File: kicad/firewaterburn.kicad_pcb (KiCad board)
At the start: 2 copper layers, 159.6 x 104.7 mm, 85 parts, among them J1 AudioJack2_SwitchT, J2 AudioJack2_SwitchT, J3 AudioJack2_SwitchT, J4 AudioJack2_SwitchT, J5 AudioJack2_SwitchT, J6 AudioJack2_SwitchT, J7 R61529 LCD, J9 Conn_01x03, P1 USB_C_Plug_USB2.0, Q1 DMN61D9UWQ-13, Q2 DMP31D0U-7, Q3 SS8050-G, Q4 SS8050-G, Q6 DMN2004WK-7, SW1 SW_MEC_5G, SW2 SW_MEC_5G, U1 RT9471GQW, U2 MCP1663T-E/MNY, U3 MCP1603-330I/MC, U4 ESP32-S3-Rx, U5 CP2102N-Axx-xQFN28

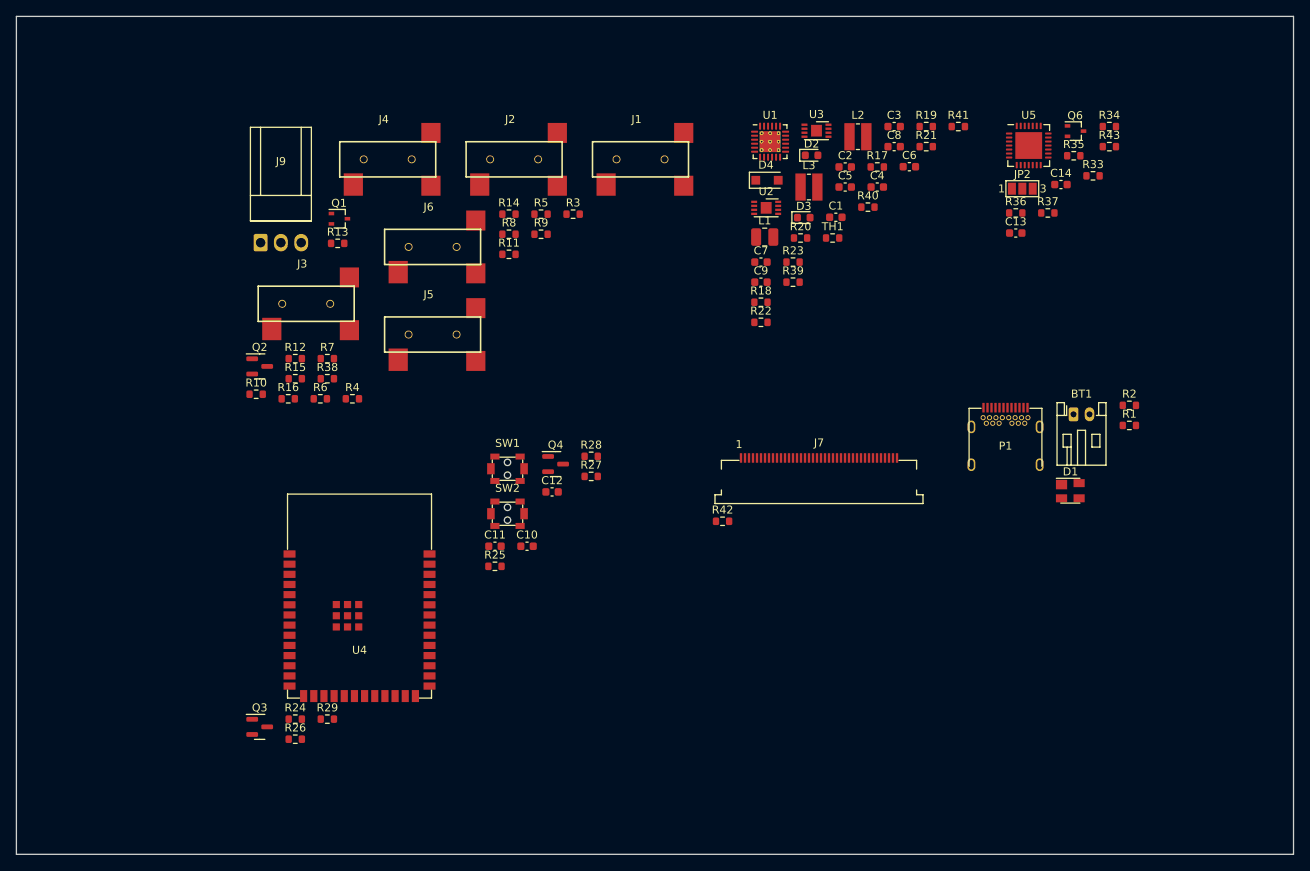
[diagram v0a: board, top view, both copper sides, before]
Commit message: route complete pcb
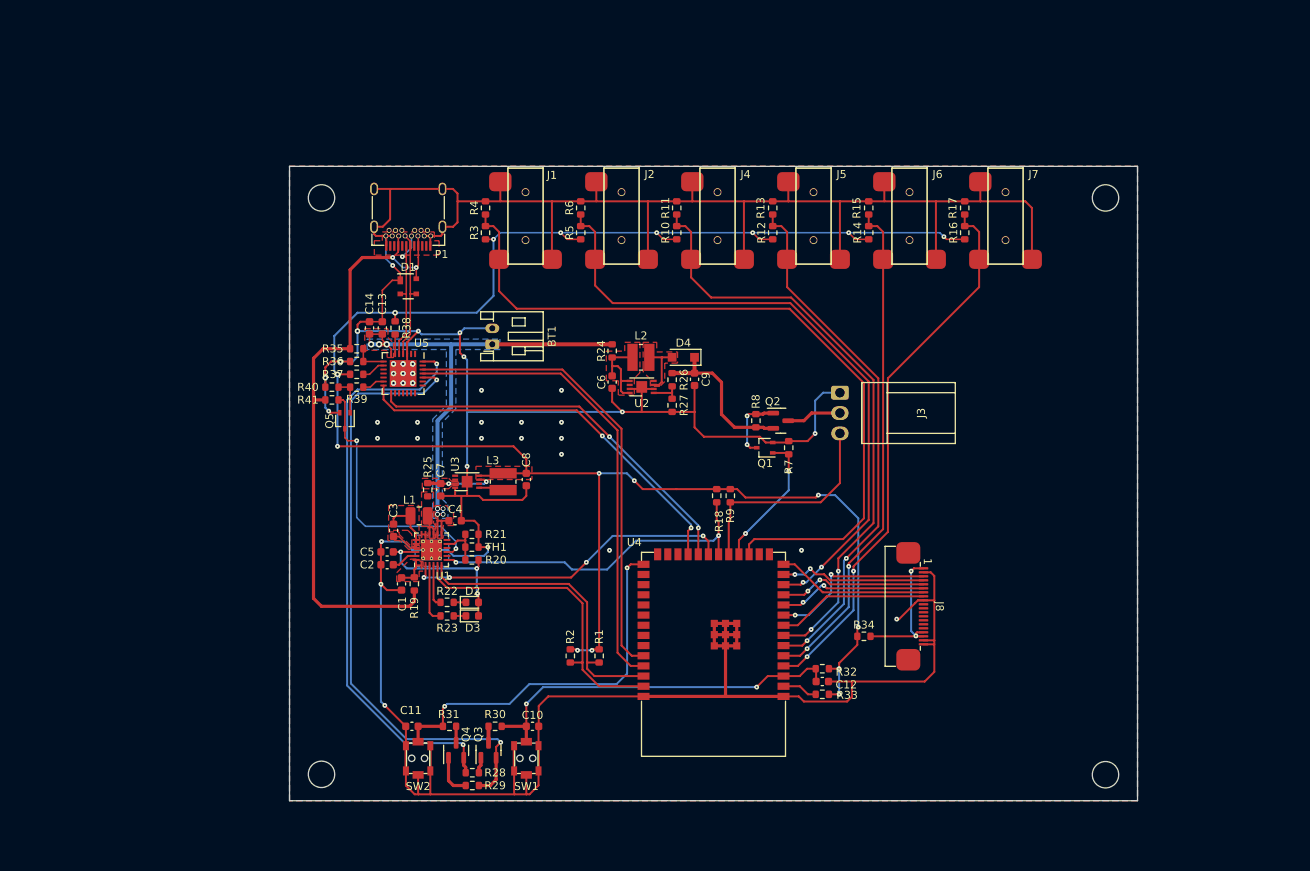
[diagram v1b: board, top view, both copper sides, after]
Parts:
- removed J9: Conn_01x03, z_connector:Molex_KK-254_AE-6410-03A_1x03_P2.54mm_Vertical
- removed JP2: SolderJumper_3_Open, Jumper:SolderJumper-3_P1.3mm_Open_Pad1.0x1.5mm_NumberLabels
- removed Q6: DMN2004WK-7, Package_TO_SOT_SMD:SOT-323_SC-70
- removed R42, R43: 0R, Resistor_SMD:R_0603_1608Metric
- added J8: R61529 LCD, z_connector:FPC_BOTTOM_20POS_Würth_68712014522, F.Cu at (176.2, 115.0)
- added Q5: DMN2004WK-7, Package_TO_SOT_SMD:SOT-323_SC-70, F.Cu at (103.9, 91.8)
- added R30: 0R, Resistor_SMD:R_0603_1608Metric, F.Cu at (122.7, 130.0)
- added R31: 0R, Resistor_SMD:R_0603_1608Metric, F.Cu at (117.0, 130.0)
- added R32: 10k, Resistor_SMD:R_0603_1608Metric, F.Cu at (163.6, 122.8)
- J3: value AudioJack2_SwitchT -> Conn_01x03; footprint z_connector:MJ-2523 -> z_connector:Molex_KK-254_AE-6410-03A_1x03_P2.54mm_Vertical
- J7: value R61529 LCD -> AudioJack2_SwitchT; footprint z_connector:62684-402100ALF -> z_connector:MJ-2523
- R10, R12: value 3k4 -> 4k42
- R11: value 4k42 -> 3k4
- R13, R17: value 10k -> 3k4
- R18: value 5k23 -> 10k
- R19: value 30k1 -> 0R
- R20: value 2k2 -> 5k23
- R21: value 2k2 -> 30k1
- R22: value 1050k -> 2k2
- R23: value 120k -> 2k2
- R24, R25: value 10k -> 0R
- R26: value 0R -> 1050k
- R27: value 0R -> 120k
- R29, R41: value 0R -> 10k
- R33: value 22k1 -> 0R
- R34: value 47k5 -> 0R
- R35: value 2k -> 22k1
- R36: value 1M -> 47k5
- R37: value 10k -> 2k
- R38: value 3k4 -> 0R
- R40: value 0R -> 1M
- R9: value 4k42 -> 10k
- U1: footprint Package_DFN_QFN:WQFN-24-1EP_4x4mm_P0.5mm_EP2.6x2.6mm_ThermalVias -> z_ic:WQFN-24-1EP_4x4mm_P0.5mm_EP2.6x2.6mm_ThermalVias
- moved R35 92.8 mm to (105.4, 82.8)
- moved R37 88.7 mm to (105.4, 86.0)
- moved C14 88.3 mm to (107.0, 80.2), turned to 90 degrees
- moved R16 87.1 mm to (181.4, 68.3), turned to 90 degrees
- moved D1 86.6 mm to (111.8, 75.0)
- moved R19 85.8 mm to (112.6, 112.2), turned to 90 degrees
- moved R41 85.4 mm to (102.3, 89.2), turned to 180 degrees
- moved R36 84.4 mm to (105.4, 84.4), turned to 180 degrees
- moved U5 83.2 mm to (111.2, 85.9), turned to -90 degrees
- moved C3 80.4 mm to (110.0, 105.5), turned to 90 degrees
- moved P1 80.4 mm to (111.8, 65.2)
- moved C13 80.1 mm to (108.6, 80.2), turned to 90 degrees
- moved R2 76.6 mm to (132.1, 121.2), turned to -90 degrees
- moved C2 75.8 mm to (109.2, 109.8), turned to 180 degrees
- moved R15 74.8 mm to (169.4, 65.2), turned to 90 degrees
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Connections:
- J4 pad T: /OUTPUT/probe5 -> /OUTPUT/probe2
- J5 pad T: /OUTPUT/probe3 -> /OUTPUT/probe5
- J6 pad T: /OUTPUT/probe6 -> /OUTPUT/probe3
- Q2 pad 3: Net-(J9-Pad2) -> Net-(J3-Pad2)
- R10 pad 1: /OUTPUT/probe2 -> +3V3
- R10 pad 2: GND -> /OUTPUT/probe2
- R11 pad 1: +3V3 -> /OUTPUT/probe2
- R11 pad 2: /OUTPUT/probe5 -> GND
- R12 pad 1: /OUTPUT/probe5 -> +3V3
- R12 pad 2: GND -> /OUTPUT/probe5
- R13 pad 1: +3V3 -> /OUTPUT/probe5
- R13 pad 2: /OUTPUT/TACHO -> GND
- R17 pad 1: /mcu_n_tft/CHR_INT -> /OUTPUT/probe6
- R17 pad 2: +3V3 -> GND
- R18 pad 1: Net-(C5-Pad1) -> /mcu_n_tft/CHR_INT
- R18 pad 2: Net-(R18-Pad2) -> +3V3
- R19 pad 1: Net-(R18-Pad2) -> VBUS
- R19 pad 2: GND -> Net-(C1-Pad1)
- R20 pad 1: Net-(D2-Pad1) -> Net-(C5-Pad1)
- R20 pad 2: /power unit/STAT -> Net-(R20-Pad2)
- R21 pad 1: Net-(D3-Pad1) -> Net-(R20-Pad2)
- R21 pad 2: /power unit/~{PG} -> GND
- R22 pad 1: +12V -> Net-(D2-Pad1)
- R22 pad 2: Net-(R22-Pad2) -> /power unit/STAT
- R23 pad 1: Net-(R22-Pad2) -> Net-(D3-Pad1)
- R23 pad 2: GND -> /power unit/~{PG}
- R24 pad 1: Net-(Q3-Pad1) -> VAA
- R24 pad 2: /USB<->UART/DTS -> Net-(C6-Pad1)
- R25 pad 1: Net-(Q4-Pad1) -> VS
- R25 pad 2: /mcu_n_tft/RTS -> Net-(C7-Pad1)
- R26 pad 1: /mcu_n_tft/EN -> +12V
- R26 pad 2: Net-(Q3-Pad3) -> Net-(R26-Pad2)
- R27 pad 1: /mcu_n_tft/BOOT -> Net-(R26-Pad2)
- R27 pad 2: Net-(Q4-Pad3) -> GND
- R28 pad 1: +3V3 -> Net-(Q3-Pad1)
- R28 pad 2: /mcu_n_tft/EN -> /USB<->UART/DTS
- R29 pad 1: Net-(R29-Pad1) -> Net-(Q4-Pad1)
- R29 pad 2: +3V3 -> /mcu_n_tft/RTS
- R33 pad 1: VBUS -> Net-(R33-Pad1)
- R33 pad 2: Net-(R33-Pad2) -> +3V3
- R34 pad 1: Net-(R33-Pad2) -> +3V3
- R34 pad 2: GND -> Net-(J8-Pad1)
- R35 pad 1: +3V3 -> VBUS
- R36 pad 1: GND -> Net-(R35-Pad2)
- R36 pad 2: Net-(Q6-Pad1) -> GND
- R37 pad 1: /USB<->UART/CHREN -> +3V3
- R37 pad 2: VBUS -> Net-(R37-Pad2)
- R38 pad 1: /OUTPUT/probe6 -> +3V3
- R38 pad 2: GND -> Net-(R38-Pad2)
- R39 pad 1: VBUS -> Net-(Q5-Pad1)
- R39 pad 2: Net-(C1-Pad1) -> /USB<->UART/CHREN_
- R40 pad 1: VAA -> GND
- R40 pad 2: Net-(C6-Pad1) -> Net-(Q5-Pad1)
- R41 pad 1: VS -> /USB<->UART/CHREN
- R41 pad 2: Net-(C7-Pad1) -> VBUS
- R9 pad 2: /OUTPUT/probe2 -> /OUTPUT/TACHO
- TH1 pad 1: Net-(R18-Pad2) -> Net-(R20-Pad2)
- U1 pad 11: Net-(R18-Pad2) -> Net-(R20-Pad2)
- U2 pad 1: Net-(R22-Pad2) -> Net-(R26-Pad2)
- U4 pad 12: /OUTPUT/probe5 -> /OUTPUT/probe4
- U4 pad 17: /OUTPUT/probe6 -> /OUTPUT/probe1
- U4 pad 18: /OUTPUT/TACHO -> /OUTPUT/PWM
- U4 pad 19: /OUTPUT/PWM -> /OUTPUT/TACHO
- U4 pad 2: Net-(R29-Pad1) -> Net-(R33-Pad1)
- U4 pad 23: /mcu_n_tft/~{PD} -> /USB<->UART/CHR1
- U4 pad 4: /OUTPUT/probe1 -> /OUTPUT/probe6
- U4 pad 5: /OUTPUT/probe2 -> /OUTPUT/probe3
- U4 pad 6: /OUTPUT/probe3 -> /OUTPUT/probe5
- U4 pad 7: /OUTPUT/probe4 -> /OUTPUT/probe2
- U4 pad 8: /USB<->UART/CHR1 -> /mcu_n_tft/~{PD}
- U5 pad 6: Net-(JP2-Pad2) -> Net-(R38-Pad2)
- U5 pad 8: Net-(R33-Pad2) -> Net-(R35-Pad2)
- U5 pad 9: Net-(R35-Pad2) -> Net-(R37-Pad2)
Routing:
- net GND: track 0.00 -> 527.7 mm, vias 0 -> 40
- net +3V3: track 0.00 -> 245.0 mm, vias 0 -> 17
- net /OUTPUT/probe1: track 0.00 -> 95.1 mm
- net /OUTPUT/probe4: track 0.00 -> 80.7 mm, vias 0 -> 2
- net VBUS: track 0.00 -> 79.0 mm, vias 0 -> 2
- net /mcu_n_tft/RTS: track 0.00 -> 78.1 mm, vias 0 -> 2
- net /OUTPUT/probe2: track 0.00 -> 75.5 mm, vias 0 -> 2
- net /USB<->UART/DTS: track 0.00 -> 72.5 mm, vias 0 -> 2
- net /OUTPUT/probe6: track 0.00 -> 69.0 mm, vias 0 -> 2
- net /OUTPUT/probe5: track 0.00 -> 66.3 mm, vias 0 -> 2
- net VAA: track 0.00 -> 65.7 mm, vias 0 -> 7
- net /OUTPUT/probe3: track 0.00 -> 62.9 mm, vias 0 -> 2
- net /USB<->UART/RXD: track 0.00 -> 59.0 mm
- net /USB<->UART/TXD: track 0.00 -> 58.3 mm
- net /USB<->UART/CHR1: track 0.00 -> 50.5 mm, vias 0 -> 2
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- added copper zone on F.Cu, net +3V3
- added copper zone on B.Cu, net GND
- added copper zone on F.Cu, net GND
- added copper zone on F.Cu, net Net-(C1-Pad1)
- added copper zone on F.Cu, net Net-(C3-Pad1)
- added copper zone on F.Cu, net Net-(C3-Pad2)
- added copper zone on F.Cu, net Net-(C6-Pad1)
- added copper zone on F.Cu, net Net-(C7-Pad1)
- added copper zone on F.Cu, net Net-(D4-Pad2)
- added copper zone on B.Cu, net VAA
- added copper zone on F.Cu, net VAA
- added copper zone on F.Cu, net VS
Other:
- board size 159.6 x 104.7 mm -> 106 x 79.3 mm
